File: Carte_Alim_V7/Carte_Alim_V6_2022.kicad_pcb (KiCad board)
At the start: 4 copper layers, 98.3 x 111.5 mm, 116 parts, among them J1 BAT_IN, J10 12VC, J11 12VC, J12 12VC, J13 12VP, J14 12VP, J15 12VP, J16 12VP, J17 12VP, J18 12VP, J19 5VC, J2 BAT_IN, J20 5V_CAN, J21 5VC, J22 5V_CAN, J23 5VC, J24 5V_CAN, J25 5VC, J26 5V_CAN, J27 5VP, J28 5VP, J29 5VP, J3 MOT_OUT, J30 5VP, J31 5VP, J32 5VP, J4 MOT_OUT, J5 MOT_OUT, J6 MOT_OUT, J7 12VC, J8 12VC, J9 12VC, U1 SIC466ED-T1-GE3, U2 TPS5450ddar, U3 SIC466ED-T1-GE3

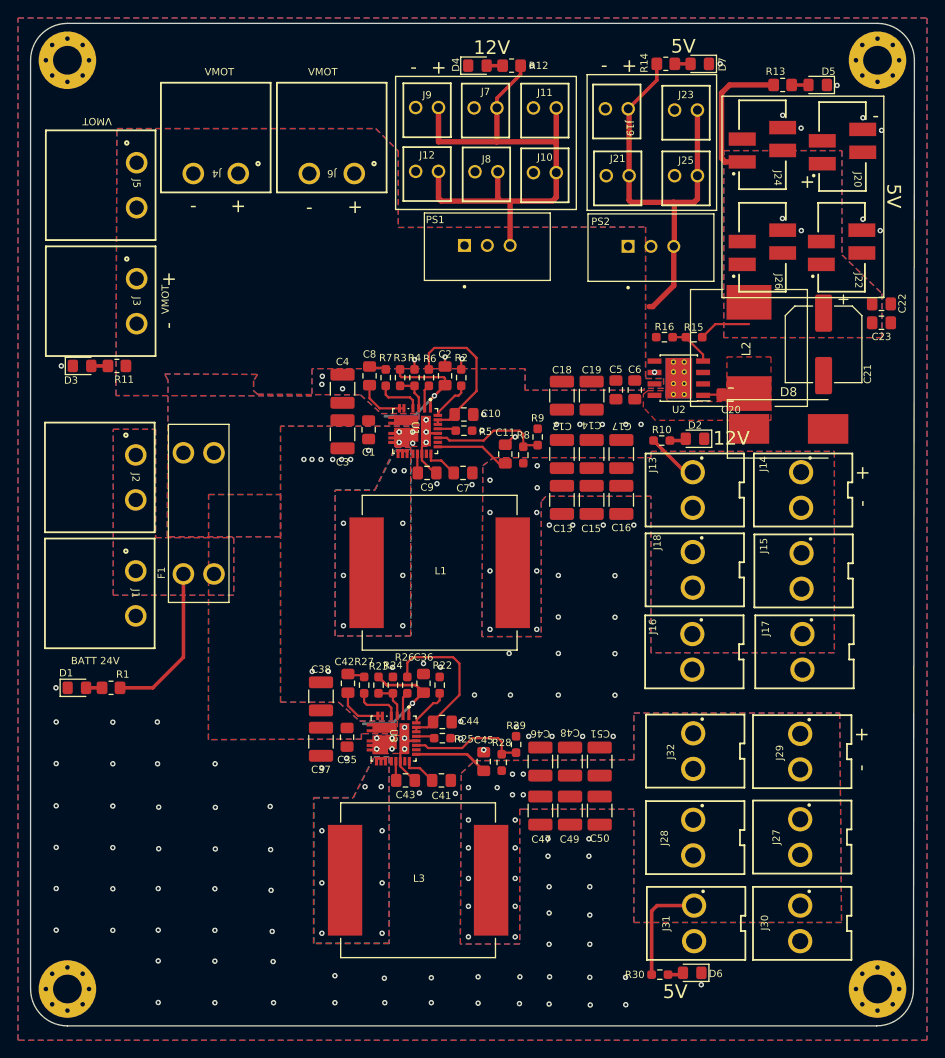
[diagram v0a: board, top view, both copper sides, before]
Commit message: update last PCBs
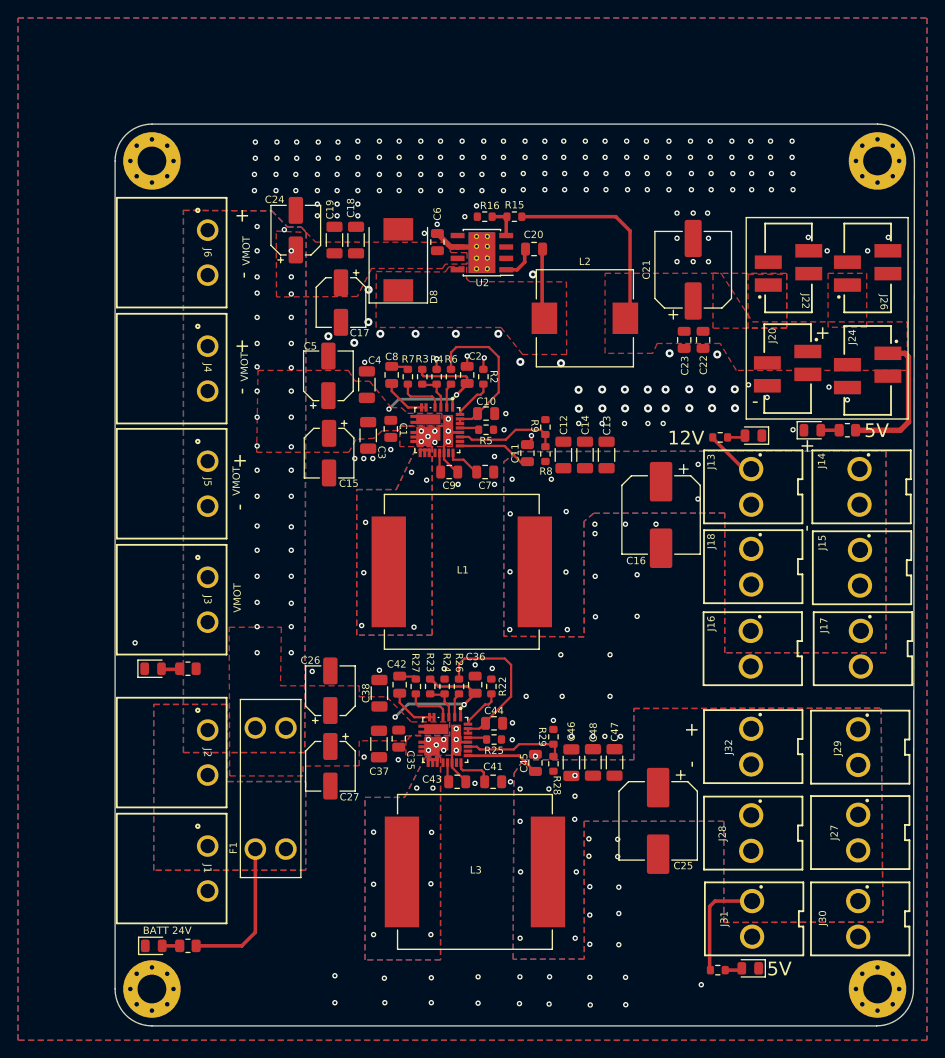
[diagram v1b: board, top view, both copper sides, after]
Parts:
- removed C49, C50, C51: 22u, Capacitor_SMD:C_1210_3225Metric_Pad1.33x2.70mm_HandSolder
- removed D4, D7: LED, LED_SMD:LED_0805_2012Metric_Pad1.15x1.40mm_HandSolder
- removed J10, J11, J12, J7, J8, J9: 12VC, AREA_lib_Connector:Wuerth_2.54mm_2pins_61900211121
- removed J19, J21, J23, J25: 5VC, AREA_lib_Connector:Wuerth_2.54mm_2pins_61900211121
- removed PS1, PS2: TSR_2-2450, AREA_lib_composant:CONV_TSR_2-2450
- removed R12: 5.1K, Resistor_SMD:R_0805_2012Metric_Pad1.20x1.40mm_HandSolder
- removed R14: 560, Resistor_SMD:R_0805_2012Metric_Pad1.20x1.40mm_HandSolder
- added C24: 10u/50V, Capacitor_SMD:CP_Elec_5x5.4, F.Cu at (75.8, 46.9)
- added C25: 330u/25V, Capacitor_SMD:CP_Elec_8x10.5, F.Cu at (116.1, 112.6)
- added C26: 10u/50V, Capacitor_SMD:CP_Elec_5x5.4, F.Cu at (79.7, 98.1)
- added C27: 10u/50V, Capacitor_SMD:CP_Elec_5x5.4, F.Cu at (79.7, 106.5)
- C1, C10, C11, C2, C20, C22, C23, C35, C36, C41, C42, C43, C44, C45, C6, C7, C8, C9: footprint Capacitor_SMD:C_0805_2012Metric_Pad1.18x1.45mm_HandSolder -> Capacitor_SMD:C_0805_2012Metric
- C12, C13, C14, C3, C37, C38, C4, C46, C47, C48: footprint Capacitor_SMD:C_1210_3225Metric_Pad1.33x2.70mm_HandSolder -> Capacitor_SMD:C_1206_3216Metric
- C15, C17: value 22u -> 10u/50V; footprint Capacitor_SMD:C_1210_3225Metric_Pad1.33x2.70mm_HandSolder -> Capacitor_SMD:CP_Elec_5x5.4
- C16: value 22u -> 330u/25V; footprint Capacitor_SMD:C_1210_3225Metric_Pad1.33x2.70mm_HandSolder -> Capacitor_SMD:CP_Elec_8x10.5
- C18, C19: value 10u -> 22u; footprint Capacitor_SMD:C_1210_3225Metric_Pad1.33x2.70mm_HandSolder -> Capacitor_SMD:C_1206_3216Metric
- C5: value 100n -> 10u/50V; footprint Capacitor_SMD:C_0805_2012Metric_Pad1.18x1.45mm_HandSolder -> Capacitor_SMD:CP_Elec_5x5.4
- D1, D2, D3, D5, D6: footprint LED_SMD:LED_0805_2012Metric_Pad1.15x1.40mm_HandSolder -> LED_SMD:LED_0805_2012Metric
- D8: footprint Diode_SMD:D_SMC_Handsoldering -> Diode_SMD:D_SMC
- L2: footprint Inductor_SMD:L_Wuerth_HCI-1335 -> Inductor_SMD:L_Wuerth_HCI-1030
- R1, R11, R13: footprint Resistor_SMD:R_0805_2012Metric_Pad1.20x1.40mm_HandSolder -> Resistor_SMD:R_0805_2012Metric
- R10, R15, R16, R2, R22, R23, R24, R25, R26, R27, R28, R29, R3, R30, R4, R5, R6, R7, R8, R9: footprint Resistor_SMD:R_0603_1608Metric_Pad0.98x0.95mm_HandSolder -> Resistor_SMD:R_0603_1608Metric
- moved D8 47.3 mm to (87.2, 50.2), turned to 90 degrees
- moved R13 39.1 mm to (137.2, 69.2), turned to 180 degrees
- moved D5 38.4 mm to (133.2, 69.2), turned to 0 degrees
- moved C17 35.4 mm to (80.8, 55.0), turned to -90 degrees
- moved D3 34.6 mm to (59.9, 95.7)
- moved R11 34.6 mm to (63.8, 95.7)
- moved J3 34.1 mm to (66.0, 88.0)
- moved J5 34.1 mm to (66.0, 75.1)
- moved C19 33.4 mm to (80.1, 48.0), turned to 90 degrees
- moved C5 32.0 mm to (79.4, 63.1), turned to 90 degrees
- moved J1 31.6 mm to (66.0, 117.9)
- moved F1 31.6 mm to (73.0, 109.0)
- moved J2 31.6 mm to (66.0, 105.0)
- moved D1 29.9 mm to (60.0, 126.5)
- moved R1 29.9 mm to (63.8, 126.5)
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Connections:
- C15 pad 1: +12P -> +24V
- C17 pad 1: +12P -> +24V
- U1 pad 30: (no net) -> GND
- U1 pad A12: (no net) -> Net-(L1-Pad1)
- U1 pad A30: (no net) -> GND
- U3 pad 30: (no net) -> GND
- U3 pad A12: (no net) -> Net-(L3-Pad1)
- U3 pad A30: (no net) -> GND
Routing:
- net +12C: track 61.2 -> 0.00 mm
- net +5C: track 47.2 -> 0.00 mm
- net +5V: track 23.4 -> 38.4 mm
- net Net-(C20-Pad1): track 0.00 -> 8.54 mm
- net GND: track 16.5 -> 22.1 mm, vias 143 -> 257
- net +24V: track 31.8 -> 35.3 mm, vias 2 -> 40
- net Net-(R28-Pad1): track 13.3 -> 11.0 mm
- net Net-(D4-Pad2): track 1.77 -> 0.00 mm
- net Net-(C20-Pad2): track 2.09 -> 3.87 mm
- net Net-(D7-Pad2): track 1.76 -> 0.00 mm
- net Net-(R8-Pad1): track 13.3 -> 11.6 mm
- net /REGULO5v/VSENS: track 4.92 -> 3.57 mm
- net +BATT: track 17.7 -> 16.4 mm
- net Net-(C41-Pad1): track 3.86 -> 4.41 mm
- net Net-(L1-Pad1): vias 8 -> 6
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- removed copper zone on B.Cu, net +5V
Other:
- board size 98.3 x 111.5 mm -> 88.9 x 100.3 mm
